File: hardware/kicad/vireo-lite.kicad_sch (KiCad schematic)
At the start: 0 parts

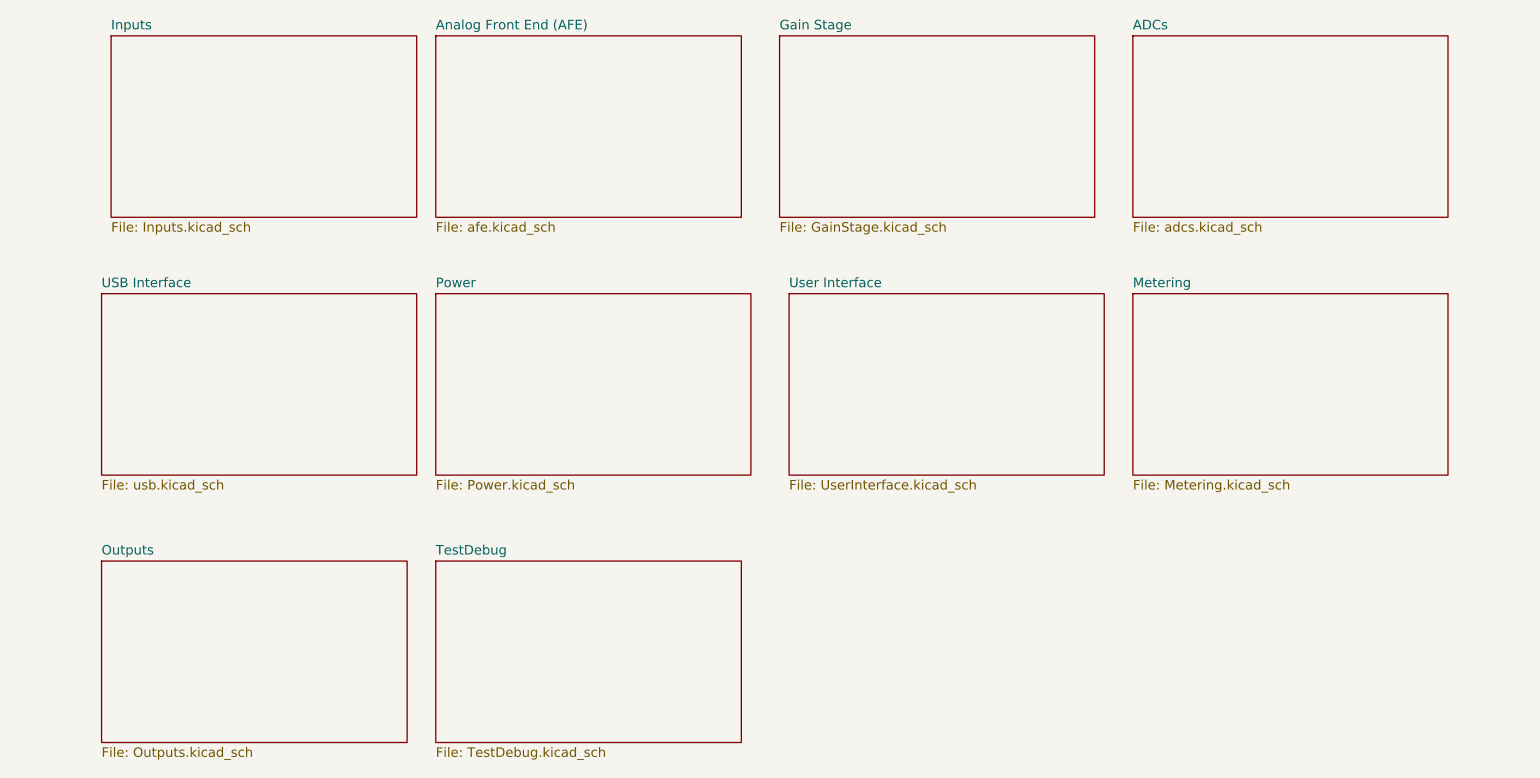
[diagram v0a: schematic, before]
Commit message: usb interface
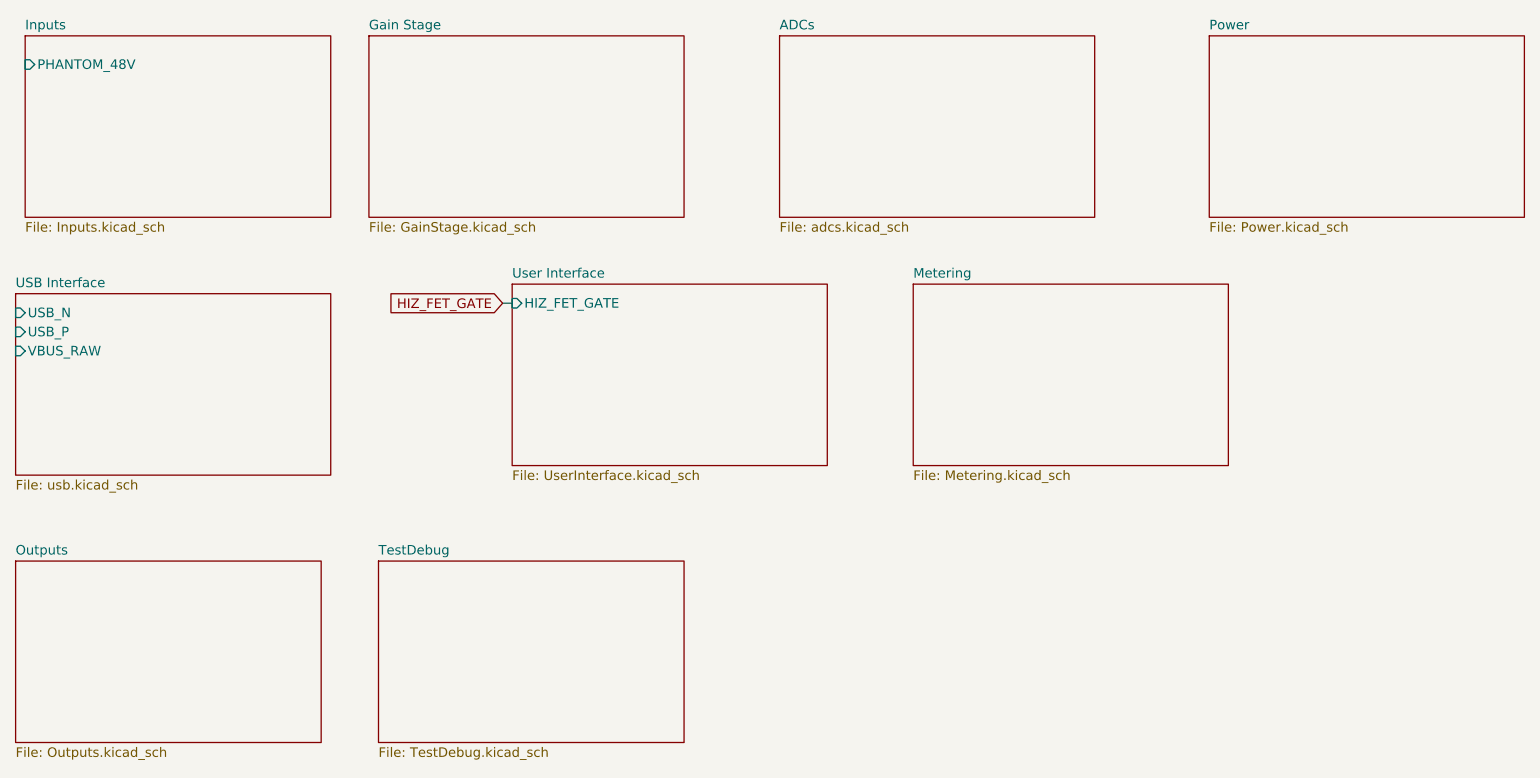
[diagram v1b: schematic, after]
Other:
- removed sheet Analog Front End (AFE)
- sheet Inputs ports: added PHANTOM_48V; removed none
- sheet USB Interface ports: added USB_N, USB_P, VBUS_RAW; removed none
- sheet User Interface ports: added HIZ_FET_GATE; removed none
